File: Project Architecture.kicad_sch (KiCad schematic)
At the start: 0 parts

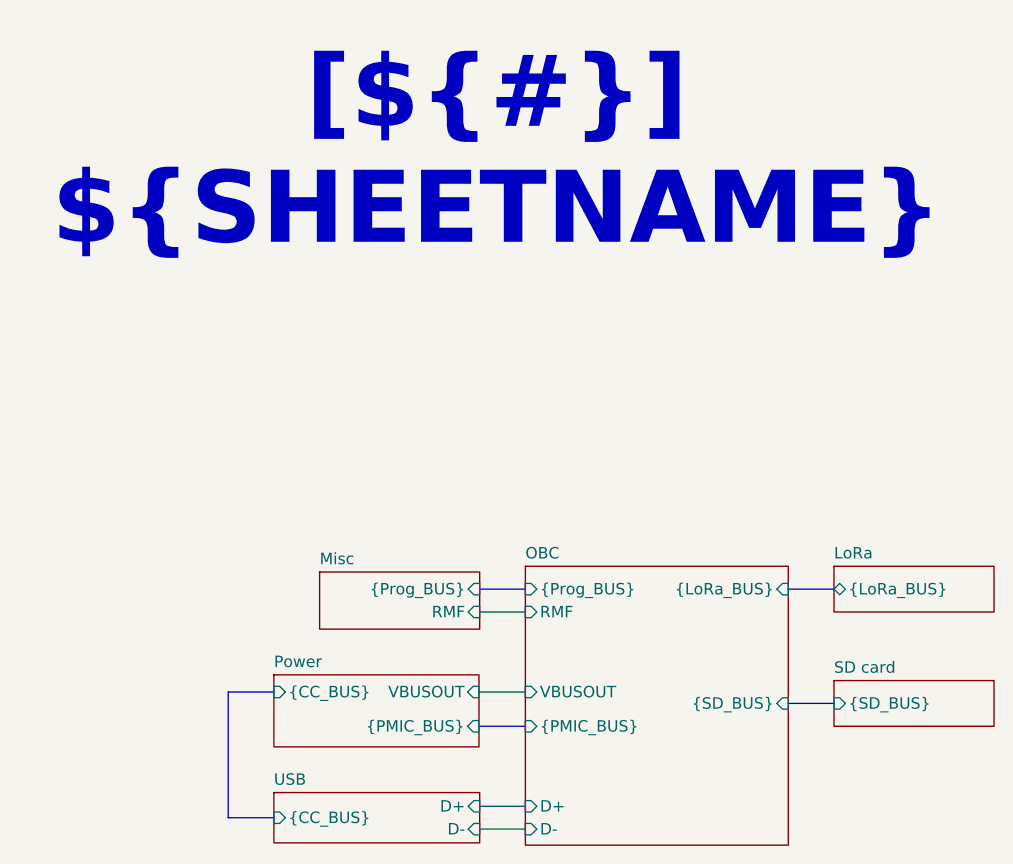
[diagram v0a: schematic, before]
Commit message: Finalized schematic
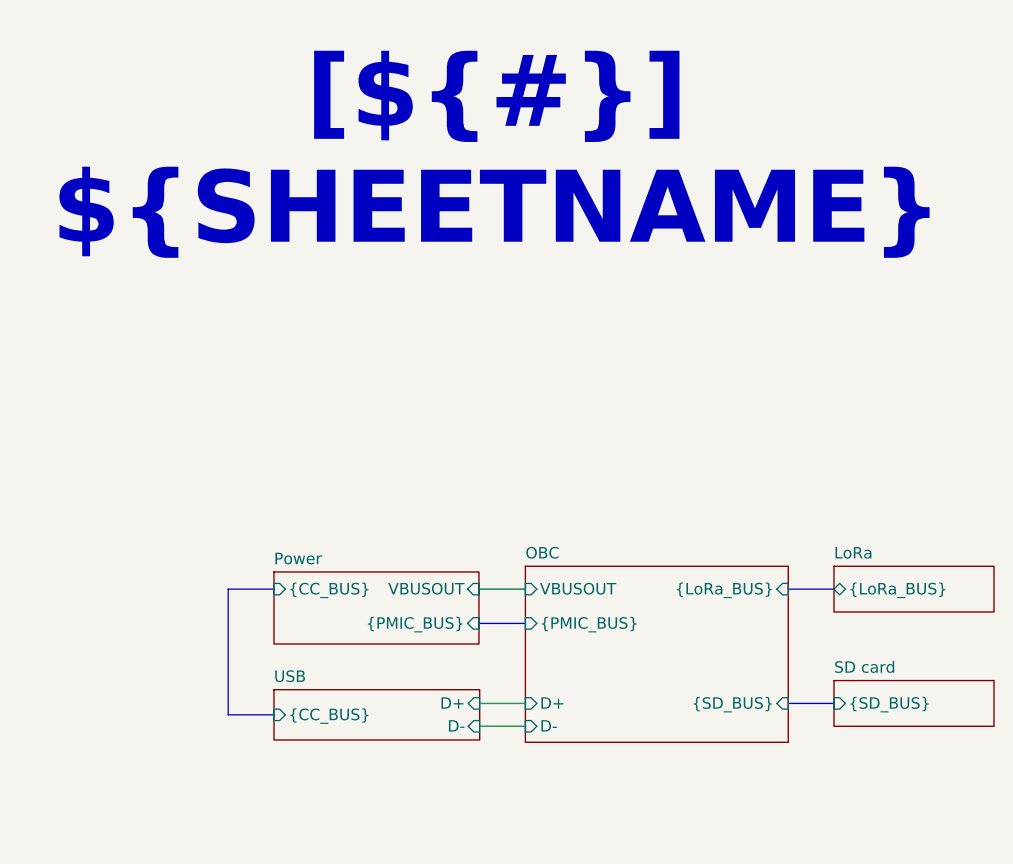
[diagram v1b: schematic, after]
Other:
- removed sheet Misc
- sheet OBC ports: added none; removed RMF, {Prog_BUS}
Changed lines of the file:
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@@
 	(wire
 		(pts
-			(xy 208.28 83.82) (xy 213.36 83.82)
+			(xy 208.28 96.52) (xy 213.36 96.52)
+		)
+		(stroke
+			(width 0)
+			(type default)
+		)
+	)
+	(bus
+		(pts
+			(xy 242.57 93.98) (xy 247.65 93.98)
+		)
+		(stroke
+			(width 0)
+			(type default)
+		)
+	)
+	(bus
+		(pts
+			(xy 180.34 81.28) (xy 180.34 95.25)
 		)
 		(stroke
@@
 	(wire
 		(pts
-			(xy 208.28 107.95) (xy 213.36 107.95)
-		)
-		(stroke
-			(width 0)
-			(type default)
-		)
-	)
-	(bus
-		(pts
-			(xy 208.28 81.28) (xy 213.36 81.28)
-		)
-		(stroke
-			(width 0)
-			(type default)
-		)
-	)
-	(bus
-		(pts
-			(xy 242.57 93.98) (xy 247.65 93.98)
-		)
-		(stroke
-			(width 0)
-			(type default)
-		)
-	)
-	(bus
-		(pts
-			(xy 180.34 92.71) (xy 180.34 106.68)
+			(xy 208.2038 81.28) (xy 213.36 81.28)
+		)
+		(stroke
+			(width 0)
+			(type default)
+		)
+	)
+	(bus
+		(pts
+			(xy 185.42 81.28) (xy 180.34 81.28)
+		)
+		(stroke
+			(width 0)
+			(type default)
+		)
+	)
+	(bus
+		(pts
+			(xy 242.57 81.28) (xy 247.65 81.28)
 		)
 		(stroke
@@
 	(wire
 		(pts
-			(xy 208.2038 92.71) (xy 213.36 92.71)
-		)
-		(stroke
-			(width 0)
-			(type default)
-		)
-	)
-	(bus
-		(pts
-			(xy 185.42 92.71) (xy 180.34 92.71)
-		)
-		(stroke
-			(width 0)
-			(type default)
-		)
-	)
-	(bus
-		(pts
-			(xy 242.57 81.28) (xy 247.65 81.28)
-		)
-		(stroke
-			(width 0)
-			(type default)
-		)
-	)
-	(wire
-		(pts
-			(xy 208.28 105.41) (xy 213.36 105.41)
-		)
-		(stroke
-			(width 0)
-			(type default)
-		)
-	)
-	(bus
-		(pts
-			(xy 180.34 106.68) (xy 185.42 106.68)
-		)
-		(stroke
-			(width 0)
-			(type default)
-		)
-	)
-	(bus
-		(pts
-			(xy 208.2038 96.52) (xy 213.36 96.52)
+			(xy 208.28 93.98) (xy 213.36 93.98)
+		)
+		(stroke
+			(width 0)
+			(type default)
+		)
+	)
+	(bus
+		(pts
+			(xy 180.34 95.25) (xy 185.42 95.25)
+		)
+		(stroke
+			(width 0)
+			(type default)
+		)
+	)
+	(bus
+		(pts
+			(xy 208.2038 85.09) (xy 213.36 85.09)
 		)
 		(stroke
@@
 	)
 	(sheet
-		(at 190.5 79.375)
-		(size 17.78 6.35)
+		(at 213.36 78.74)
+		(size 29.21 19.558)
 		(exclude_from_sim no)
 		(in_bom yes)
@@
 		)
 		(fill
-			(color 0 255 255 1)
-		)
-		(property "Sheetname" "Misc"
-			(at 190.5 78.6634 0)
-			(show_name no)
-			(do_not_autoplace no)
-			(effects
-				(font
-					(size 1.27 1.27)
-				)
-				(justify left bottom)
-			)
-		)
-		(property "Sheetfile" "Misc.kicad_sch"
-			(at 190.5 86.3096 0)
-			(hide yes)
-			(show_name no)
-			(do_not_autoplace no)
-			(effects
-				(font
-					(size 1.27 1.27)
-				)
-				(justify left top)
-			)
-		)
-		(pin "{Prog_BUS}" input
-			(at 208.28 81.28 0)
-			(effects
-				(font
-					(size 1.27 1.27)
-				)
-				(justify right)
-			)
-		)
-		(pin "RMF" input
-			(at 208.28 83.82 0)
-			(effects
-				(font
-					(size 1.27 1.27)
-				)
-				(justify right)
-			)
-		)
-		(instances
-			(project "CanSat_Devboard"
-				(path "/f9e05184-c88b-4a88-ae9c-ab2bdb32be7c/5d00bd0a-3bbf-46b2-b8c5-f75441fb4350"
-					(page "7")
-				)
-			)
-		)
-	)
-	(sheet
-		(at 213.36 78.74)
-		(size 29.21 30.988)
-		(exclude_from_sim no)
-		(in_bom yes)
-		(on_board yes)
-		(dnp no)
-		(fields_autoplaced yes)
-		(stroke
-			(width 0.1524)
-			(type solid)
-		)
-		(fill
 			(color 255 229 191 1)
 		)
@@
 		)
 		(property "Sheetfile" "OBC.kicad_sch"
-			(at 213.36 110.3126 0)
+			(at 213.36 98.8826 0)
 			(hide yes)
 			(show_name no)
@@
 		)
 		(pin "D+" input
-			(at 213.36 105.41 180)
+			(at 213.36 93.98 180)
 			(effects
 				(font
@@
 		)
 		(pin "D-" input
-			(at 213.36 107.95 180)
+			(at 213.36 96.52 180)
 			(effects
 				(font
@@
 			)
 		)
-		(pin "{Prog_BUS}" input
+		(pin "VBUSOUT" input
 			(at 213.36 81.28 180)
 			(effects
@@
 			)
 		)
-		(pin "RMF" input
-			(at 213.36 83.82 180)
-			(effects
-				(font
-					(size 1.27 1.27)
-				)
-				(justify left)
-			)
-		)
-		(pin "VBUSOUT" input
-			(at 213.36 92.71 180)
-			(effects
-				(font
-					(size 1.27 1.27)
-				)
-				(justify left)
-			)
-		)
 		(pin "{PMIC_BUS}" input
-			(at 213.36 96.52 180)
+			(at 213.36 85.09 180)
 			(effects
 				(font
@@
 	)
 	(sheet
-		(at 185.42 103.886)
+		(at 185.42 92.456)
 		(size 22.86 5.588)
 		(exclude_from_sim no)
@@
 		)
 		(property "Sheetname" "USB"
-			(at 185.42 103.1744 0)
+			(at 185.42 91.7444 0)
 			(show_name no)
 			(do_not_autoplace no)
@@
 		)
 		(property "Sheetfile" "USB.kicad_sch"
-			(at 185.42 110.0586 0)
+			(at 185.42 98.6286 0)
 			(hide yes)
 			(show_name no)
@@
 		)
 		(pin "D+" input
-			(at 208.28 105.41 0)
+			(at 208.28 93.98 0)
 			(effects
 				(font
@@
 		)
 		(pin "D-" input
-			(at 208.28 107.95 0)
+			(at 208.28 96.52 0)
 			(effects
 				(font
@@
 		)
 		(pin "{CC_BUS}" input
-			(at 185.42 106.68 180)
+			(at 185.42 95.25 180)
 			(effects
 				(font
@@
 	)
 	(sheet
-		(at 185.42 90.8049)
+		(at 185.42 79.3749)
 		(size 22.7838 8.0011)
 		(exclude_from_sim no)
@@
 		)
 		(property "Sheetname" "Power"
-			(at 185.42 90.0933 0)
+			(at 185.42 78.6633 0)
 			(show_name no)
 			(do_not_autoplace no)
@@
 		)
 		(property "Sheetfile" "Power.kicad_sch"
-			(at 185.42 99.3906 0)
+			(at 185.42 87.9606 0)
 			(hide yes)
 			(show_name no)
@@
 		)
 		(pin "VBUSOUT" input
-			(at 208.2038 92.71 0)
+			(at 208.2038 81.28 0)
 			(effects
 				(font
@@
 		)
 		(pin "{PMIC_BUS}" input
-			(at 208.2038 96.52 0)
+			(at 208.2038 85.09 0)
 			(effects
 				(font
@@
 		)
 		(pin "{CC_BUS}" input
-			(at 185.42 92.71 180)
-			(effects
-				(font
+			(at 185.42 81.28 180)
+			(effects
+				(font
